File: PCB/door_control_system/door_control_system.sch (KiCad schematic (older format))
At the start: 74 parts, among them J1 Conn_02x06_Top_Bottom, J2 Conn_02x06_Top_Bottom, J3 Conn_02x06_Top_Bottom, J4 Barrel_Jack, J5 Screw_Terminal_01x02, K1 DIPxx-1Axx-13x, Q1 2N7000, Q10 BSS84, Q11 BSS84, Q12 BSS84, Q13 BSS84, Q2 2N7000, Q3 2N7000, Q4 2N7000, Q5 2N7000, Q6 2N7000, Q7 2N7000, Q8 2N7000, Q9 2N7000, SW1 SW_MEC_5G, SW10 SW_MEC_5G, SW11 SW_MEC_5G, SW12 SW_MEC_5G, SW13 SW_MEC_5G, SW2 SW_MEC_5G, SW3 SW_MEC_5G, SW4 SW_MEC_5G, SW5 SW_MEC_5G, SW6 SW_MEC_5G, SW7 SW_MEC_5G, SW8 SW_MEC_5G, SW9 SW_MEC_5G, U1 HDSP-A401, U2 HDSP-A401, U3 HDSP-A401, U4 HDSP-A401

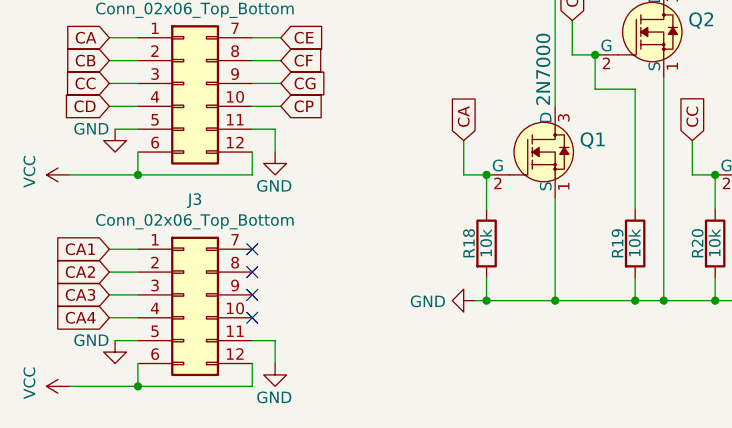
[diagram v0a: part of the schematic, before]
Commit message: Update readme
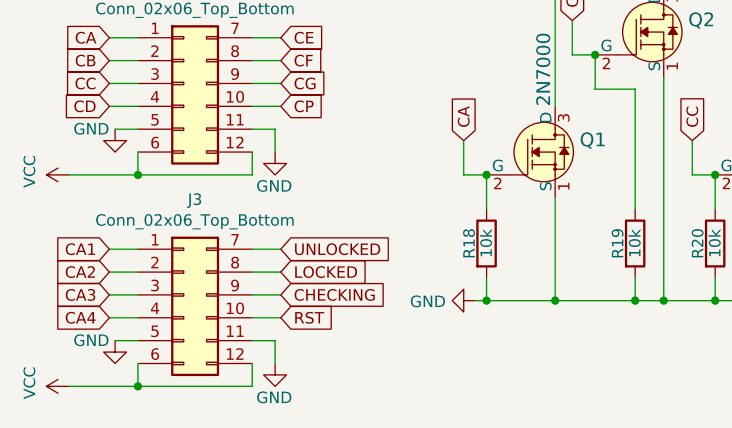
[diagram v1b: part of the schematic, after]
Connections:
- net CHECKING: now also J3.9 (Pin_9)
- net LOCKED: now also J3.8 (Pin_8)
- net RST: now also J3.10 (Pin_10)
- net UNLOCKED: now also J3.7 (Pin_7)
- no-connect marks 4 -> 0
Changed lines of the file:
@@
 Text GLabel 1075 7225 0    50   Input ~ 0
 CA4
-NoConn ~ 1700 6925
-NoConn ~ 1700 7025
-NoConn ~ 1700 7125
-NoConn ~ 1700 7225
 $Comp
 L Device:R R25
@@
 Wire Wire Line
 	2400 4650 2575 4650
+Text GLabel 1825 7225 2    50   Input ~ 0
+RST
+Text GLabel 1825 7025 2    50   Input ~ 0
+LOCKED
+Text GLabel 1825 6925 2    50   Input ~ 0
+UNLOCKED
+Text GLabel 1825 7125 2    50   Input ~ 0
+CHECKING
+Wire Wire Line
+	1700 7225 1825 7225
+Wire Wire Line
+	1700 7125 1825 7125
+Wire Wire Line
+	1700 7025 1825 7025
+Wire Wire Line
+	1700 6925 1825 6925
 $EndSCHEMATC
